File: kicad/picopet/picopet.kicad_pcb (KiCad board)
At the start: 2 copper layers, 54.8 x 37.7 mm, 59 parts, among them J1 USB_C_Receptacle_USB2.0_14P, J2 MicroJST 1.25mm female, J3 CR1220 Holder, J4 ST7735 LCD, M1 Motor_DC, Q1 SS8050, SW1 PWR, SW2 BOOTSEL, SW4 Btn0, SW5 Btn1, SW6 Btn2, SW7 Btn3, U1 RP2040, U2 MCP73831-2-OT, U3 S-T111B33MC-OGSTFU, U4 DS3231MZ, U6 AT24CS32-SSHM, U7 W25Q128JVS, Y1 ABLS-12.000MHZ-B4-T

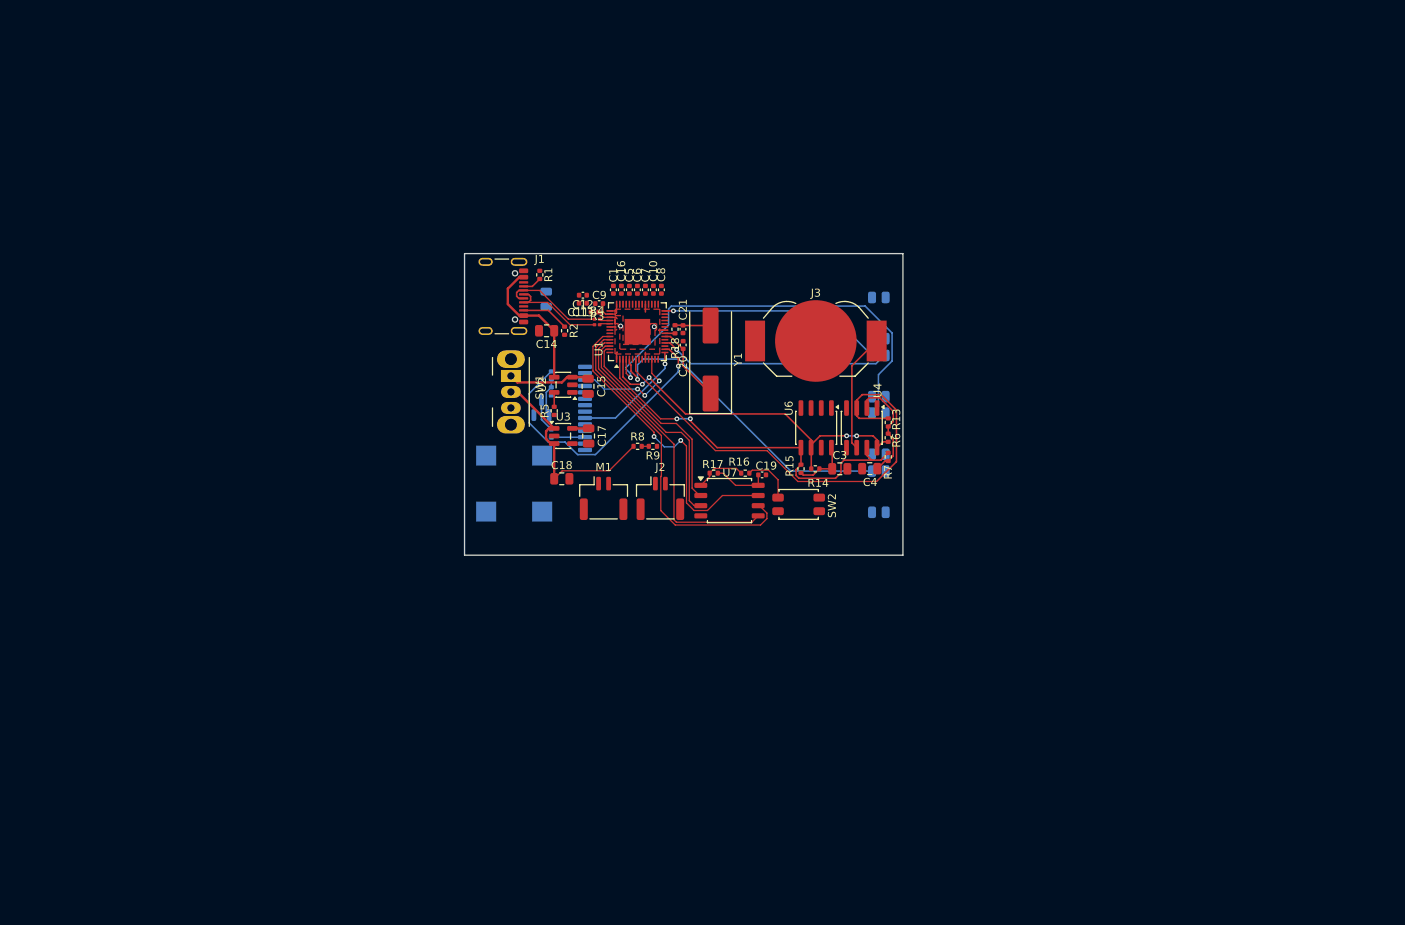
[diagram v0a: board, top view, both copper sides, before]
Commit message: Redesigning pcb
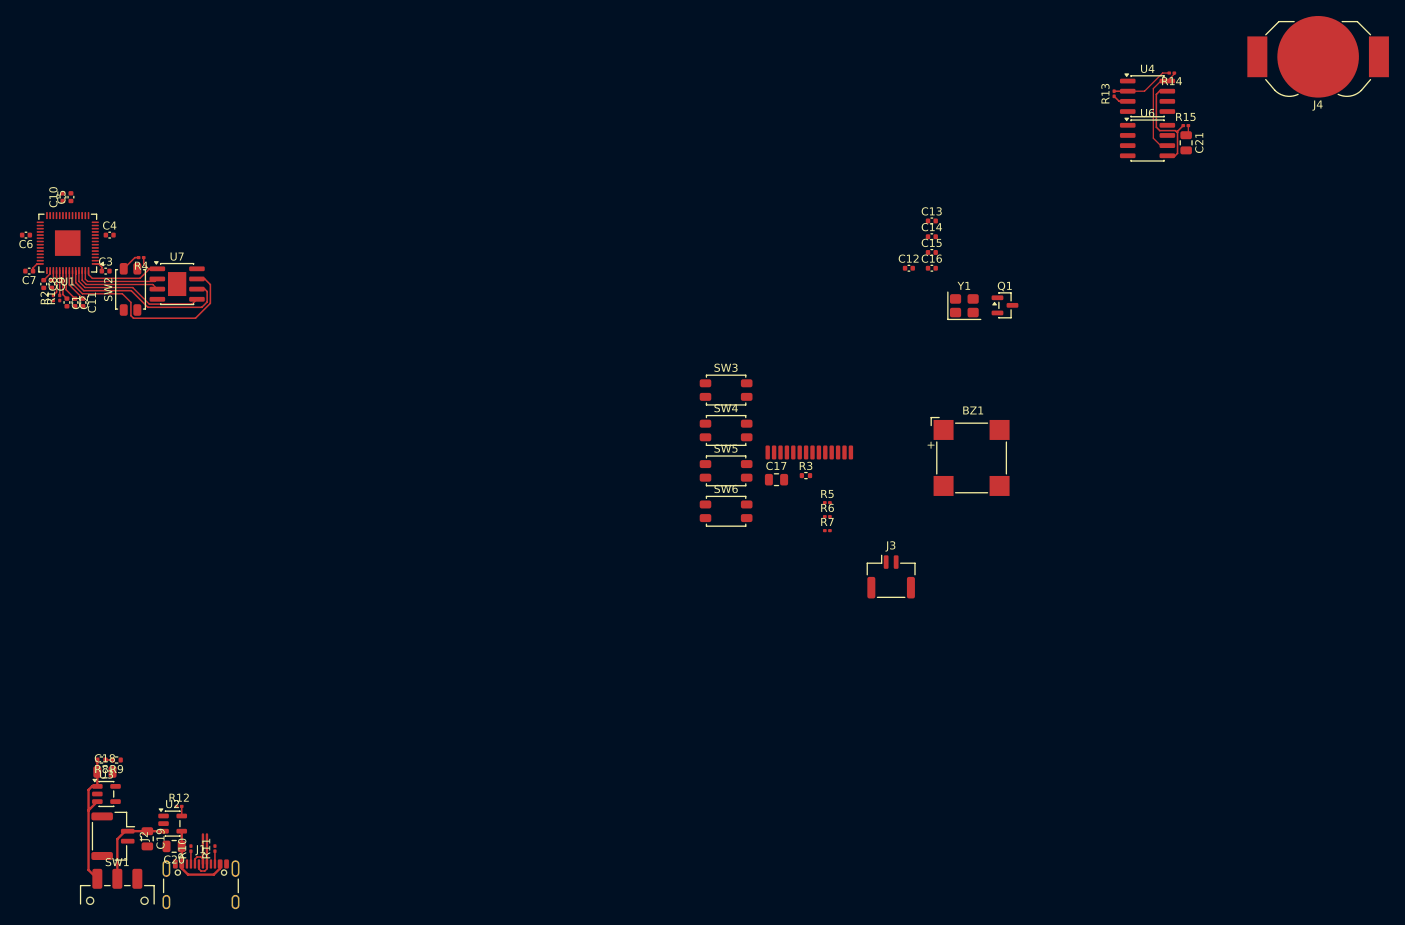
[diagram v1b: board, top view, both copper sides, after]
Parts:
- removed M1: Motor_DC, Connector_JST:JST_GH_SM02B-GHS-TB_1x02-1MP_P1.25mm_Horizontal
- removed R16, R18: 1k, Resistor_SMD:R_0402_1005Metric
- removed R17: DNF, Resistor_SMD:R_0402_1005Metric
- removed SW7: Btn3, Button_Switch_SMD:SW_SPST_EVQP2_MiddlePushTravel_H2.5mm
- added J5: ST7735 LCD, custom:ST7735_P0.8mm, F.Cu at (115.4, 58.5)
- added SW3: Btn0, Button_Switch_SMD:SW_SPST_EVQP2_MiddlePushTravel_H2.5mm, F.Cu at (105.1, 65.4)
- BZ1, Q1: moved to F.Cu
- C11: value 1u -> 100n
- C12, C13: value 100n -> 15p
- C14, C3, C4: value 4.7u -> 100n; footprint Capacitor_SMD:C_0805_2012Metric -> Capacitor_SMD:C_0402_1005Metric
- C15: value 4.7u -> 2u2; footprint Capacitor_SMD:C_0805_2012Metric -> Capacitor_SMD:C_0402_1005Metric
- C16, C8: value 100n -> 1u
- C19: value 100n -> 4.7u; footprint Capacitor_SMD:C_0402_1005Metric -> Capacitor_SMD:C_0805_2012Metric
- C2: value 1u -> 100n; footprint Capacitor_SMD:C_0805_2012Metric -> Capacitor_SMD:C_0402_1005Metric; moved to F.Cu
- C20, C21: value 27p -> 4.7u; footprint Capacitor_SMD:C_0402_1005Metric -> Capacitor_SMD:C_0805_2012Metric
- J2: value MicroJST 1.25mm female -> PH1.25mm 2P
- J3: value CR1220 Holder -> PH1.25mm 2P; footprint Battery:BatteryHolder_LINX_BAT-HLD-012-SMT -> Connector_JST:JST_GH_SM02B-GHS-TB_1x02-1MP_P1.25mm_Horizontal
- J4: value ST7735 LCD -> CR1220 Holder; footprint custom:ST7735_P0.8mm -> Battery:BatteryHolder_LINX_BAT-HLD-012-SMT; moved to F.Cu
- R1, R2: value 5K1 -> 27; footprint Resistor_SMD:R_0402_1005Metric -> Resistor_SMD:R_0201_0603Metric
- R10: value 10 -> 5k1; footprint Resistor_SMD:R_0402_1005Metric -> Resistor_SMD:R_0201_0603Metric; moved to F.Cu
- R11: value 10K -> 5k1; footprint Resistor_SMD:R_0402_1005Metric -> Resistor_SMD:R_0201_0603Metric; moved to F.Cu
- R12: value 1K -> 5k1; footprint Resistor_SMD:R_0402_1005Metric -> Resistor_SMD:R_0201_0603Metric; moved to F.Cu
- R13, R14, R15: footprint Resistor_SMD:R_0402_1005Metric -> Resistor_SMD:R_0201_0603Metric
- R3: value 27 -> 1k; footprint Resistor_SMD:R_0201_0603Metric -> Resistor_SMD:R_0402_1005Metric
- R4: value 27 -> 1k
- R5: value 5K1 -> 10; footprint Resistor_SMD:R_0402_1005Metric -> Resistor_SMD:R_0201_0603Metric
- R6: value 5K1 -> 10k; footprint Resistor_SMD:R_0402_1005Metric -> Resistor_SMD:R_0201_0603Metric
- R7: value 5K1 -> 1k; footprint Resistor_SMD:R_0402_1005Metric -> Resistor_SMD:R_0201_0603Metric
- SW1: footprint Button_Switch_THT:SW_Slide_SPDT_Angled_CK_OS102011MA1Q -> Button_Switch_SMD:SW_SPDT_CK_JS102011SAQN
- SW4: value Btn0 -> Btn1; moved to F.Cu
- SW5: value Btn1 -> Btn2; moved to F.Cu
- SW6: value Btn2 -> Btn3; moved to F.Cu
- U7: value W25Q128JVS -> W25Q32JVSSIQ; footprint Package_SO:SOIC-8_5.3x5.3mm_P1.27mm -> Package_SO:SOIC-8-1EP_3.9x4.9mm_P1.27mm_EP2.29x3mm
- Y1: value ABLS-12.000MHZ-B4-T -> X322512MSB4SI; footprint Crystal:Crystal_SMD_HC49-SD -> Crystal:Crystal_SMD_3225-4Pin_3.2x2.5mm
- moved C4 99.4 mm to (28.0, 46.0), turned to 0 degrees
- moved C3 95.0 mm to (27.5, 50.5)
- moved C20 89.3 mm to (36.1, 122.4), turned to 180 degrees
- moved C19 89.3 mm to (32.8, 121.5), turned to -90 degrees
- moved J4 88.7 mm to (179.1, 23.7), turned to 0 degrees
- moved SW2 87.7 mm to (30.6, 52.8), turned to 90 degrees
- moved J1 83.1 mm to (39.5, 128.3), turned to 0 degrees
- moved SW1 82.0 mm to (29.0, 129.2), turned to 0 degrees
- moved J2 80.4 mm to (28.4, 121.1), turned to -90 degrees
- moved R9 77.7 mm to (28.9, 111.6)
- moved R8 77.7 mm to (27.0, 111.6)
- moved C8 77.2 mm to (19.8, 52.1), turned to -90 degrees
- moved C7 77.1 mm to (18.0, 50.5), turned to 180 degrees
- moved C6 76.7 mm to (17.6, 46.0), turned to 180 degrees
- moved C10 74.7 mm to (22.2, 41.2)
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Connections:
- net GPIO_UNDECIDE_B renamed GPIO26
- C10 pad 1: +3V3 -> +1V1
- C12 pad 1: +1V1 -> /XIN
- C13 pad 1: +1V1 -> Net-(C13-Pad1)
- C14 pad 1: Net-(U2-V_{DD}) -> +3V3
- C15 pad 1: VBAT -> GND
- C15 pad 2: GND -> +3V3
- C16 pad 1: +3V3 -> GND
- C16 pad 2: GND -> +3V3
- C19 pad 1: +3V3 -> VBAT
- C20 pad 1: /XIN -> USBC_VDD
- C21 pad 1: Net-(C21-Pad1) -> +3V3
- C9 pad 1: +3V3 -> +1V1
- J1 pad A4: Net-(U2-V_{DD}) -> USBC_VDD
- J1 pad A9: Net-(U2-V_{DD}) -> USBC_VDD
- J1 pad B4: Net-(U2-V_{DD}) -> USBC_VDD
- J1 pad B9: Net-(U2-V_{DD}) -> USBC_VDD
- J3 pad 1: VCOIN -> GND
- J3 pad 2: GND -> GPIO6
- J4 pad 1: (no net) -> VCOIN
- R1 pad 1: Net-(J1-CC1) -> USB_D+
- R1 pad 2: GND -> Net-(U1-USB_DP)
- R10 pad 1: Net-(J4-LED-) -> Net-(J1-CC1)
- R10 pad 2: Net-(Q1-C) -> GND
- R11 pad 1: +3V3 -> Net-(J1-CC2)
- R11 pad 2: Net-(Q1-B) -> GND
- R12 pad 1: Net-(Q1-B) -> GND
- R12 pad 2: GPIO13 -> Net-(U2-PROG)
- R2 pad 1: Net-(J1-CC2) -> USB_D-
- R2 pad 2: GND -> Net-(U1-USB_DM)
- R3 pad 1: USB_D+ -> /XOUT
- R3 pad 2: Net-(U1-USB_DP) -> Net-(C13-Pad1)
- R4 pad 1: USB_D- -> /QSPI_SS
- R4 pad 2: Net-(U1-USB_DM) -> Net-(R4-Pad2)
- R5 pad 1: GND -> Net-(Q1-C)
- R5 pad 2: Net-(U2-PROG) -> Net-(J5-LED-)
- R6 pad 1: GPIO1 -> Net-(Q1-B)
- R7 pad 1: GPIO0 -> GPIO13
- R7 pad 2: +3V3 -> Net-(Q1-B)
- SW1 pad 1: VBAT -> VSENSE
- SW1 pad 2: VSENSE -> VBAT
- SW1 pad 3: (no net) -> unconnected-(SW1-C-Pad3)
- SW2 pad 1: GND -> Net-(R4-Pad2)
- SW2 pad 2: Net-(R16-Pad2) -> GND
- SW4 pad 1: GPIO15 -> GPIO17
- SW5 pad 1: GPIO17 -> GPIO2
- SW6 pad 1: GPIO2 -> GPIO3
- U1 pad 37: /GPIO25 -> GPIO25
- U2 pad 1: GPIO_UNDECIDE_A -> GPIO25
- U2 pad 4: Net-(U2-V_{DD}) -> USBC_VDD
- Y1 pad 2: Net-(C21-Pad1) -> Net-(C13-Pad1)
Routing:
- net GPIO5: track 59.3 -> 1.96 mm
- net GPIO2: track 54.1 -> 0.00 mm, vias 1 -> 0
- net GPIO3: track 40.2 -> 0.00 mm, vias 1 -> 0
- net GPIO13: track 36.0 -> 0.00 mm, vias 1 -> 0
- net GPIO0: track 48.1 -> 14.1 mm, vias 2 -> 0
- net GPIO1: track 45.3 -> 11.8 mm, vias 4 -> 0
- net GPIO15: track 31.0 -> 0.00 mm, vias 1 -> 0
- net GPIO17: track 28.2 -> 0.00 mm, vias 1 -> 0
- net /QSPI_SD0: track 38.0 -> 17.5 mm
- net /QSPI_SCLK: track 42.5 -> 22.6 mm
- net +3V3: track 40.0 -> 21.3 mm
- net Net-(U2-V_{DD}): track 17.5 -> 0.00 mm
- net /QSPI_SD2: track 27.5 -> 11.1 mm
- net VCOIN: track 14.9 -> 0.00 mm
- net /QSPI_SD1: track 25.1 -> 10.3 mm
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- removed copper zone on F.Cu, net +1V1
- removed copper zone on F.Cu, net +3V3
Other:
- board outline removed
